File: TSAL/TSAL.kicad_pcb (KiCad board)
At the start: 2 copper layers, 89.4 x 58.2 mm, 58 parts, among them J1 Conn_02x03_Counter_Clockwise, J2 Conn_01x02, J3 Conn_02x01, J4 Conn_02x01, Q1 BSS138, Q2 BSS138, Q3 AO3401A, U1 LM358, U10 74HC74, U2 74HC27, U3 74HC20, U4 4N35, U5 74HC08, U6 74HC86, U7 LM7805_TO220, U8 LM339, U9 LM339

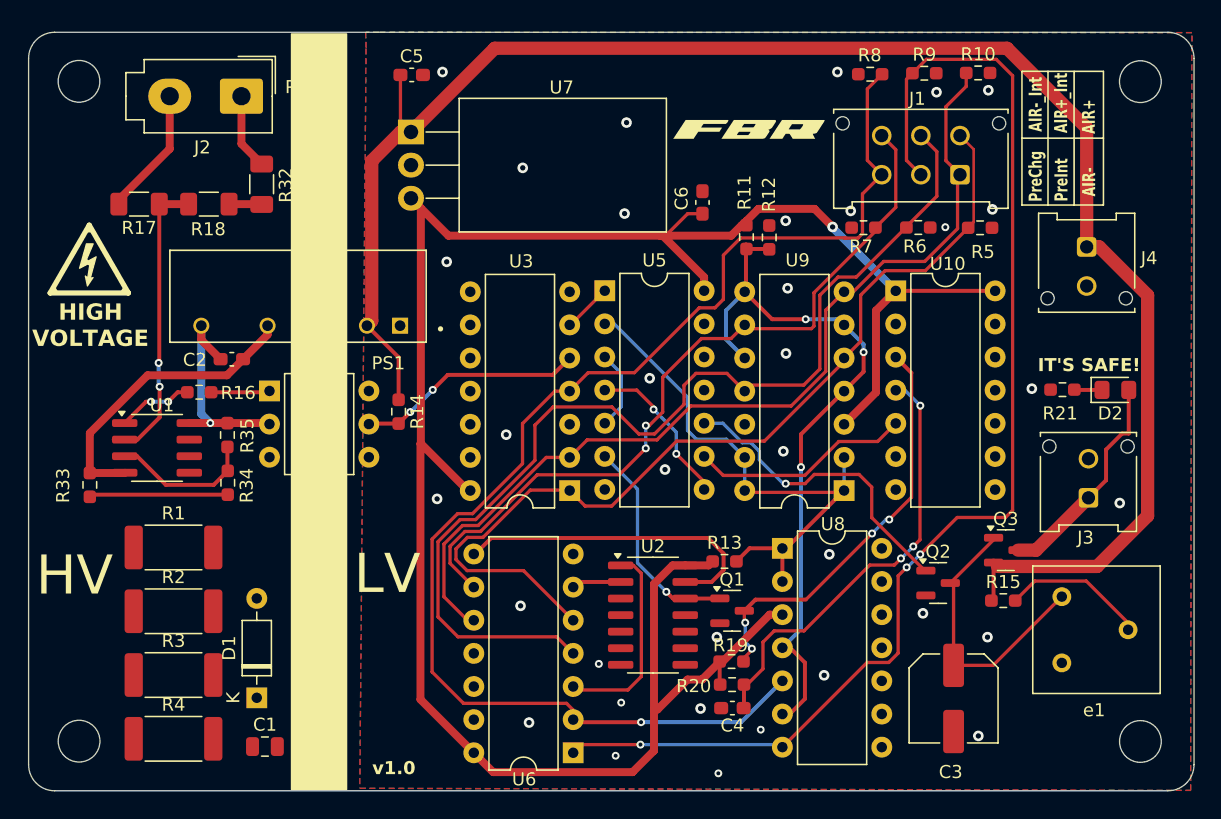
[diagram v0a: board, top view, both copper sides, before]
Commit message: minor changes
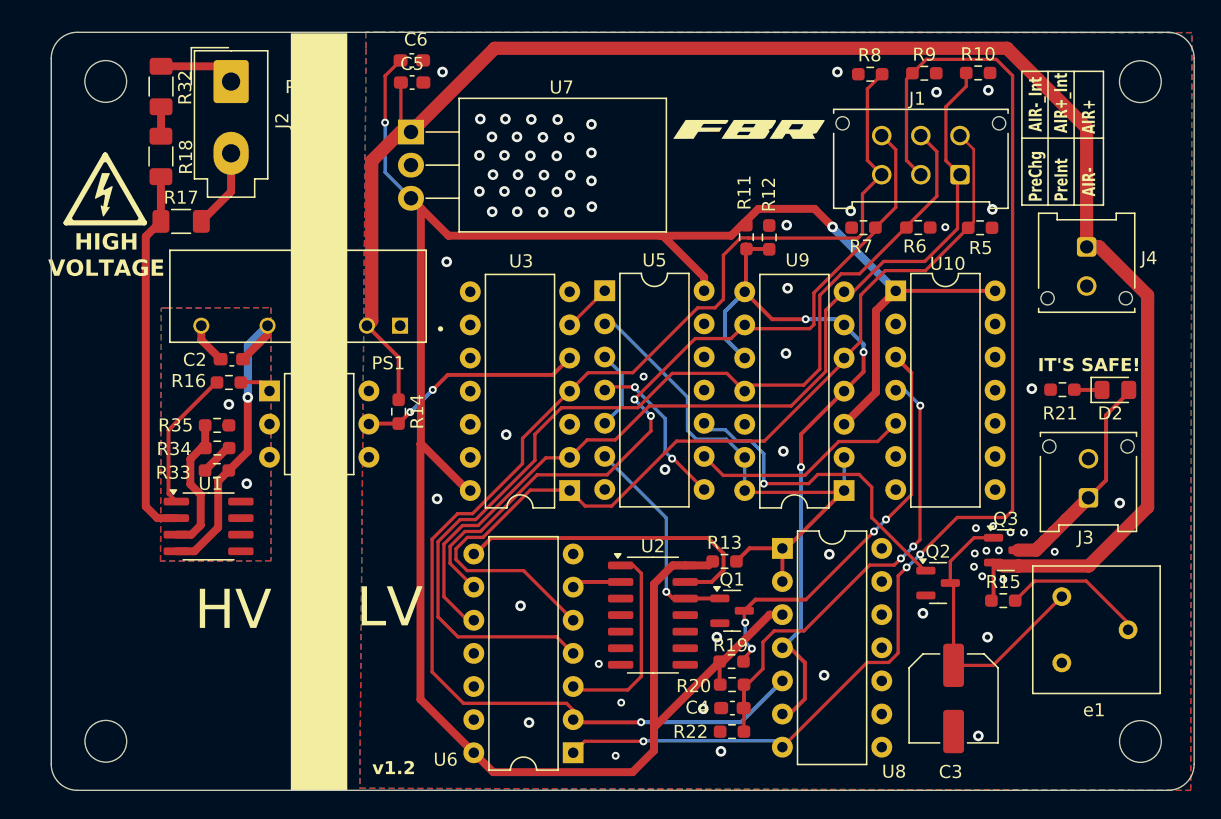
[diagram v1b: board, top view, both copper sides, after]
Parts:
- removed C1: 0.1 uF, Capacitor_SMD:C_0805_2012Metric
- removed D1: 2.4V, Diode_THT:D_DO-35_SOD27_P7.62mm_Horizontal
- removed R1, R2: 5.6K, Resistor_SMD:R_2512_6332Metric_Pad1.40x3.35mm_HandSolder
- removed R3: 6.8K, Resistor_SMD:R_2512_6332Metric_Pad1.40x3.35mm_HandSolder
- removed R4: 2.7K, Resistor_SMD:R_2512_6332Metric_Pad1.40x3.35mm_HandSolder
- added R22: 500K, Resistor_SMD:R_0603_1608Metric_Pad0.98x0.95mm_HandSolder, F.Cu at (112.4, 84.4)
- R16: value 500 -> 390
- moved C6 24.8 mm to (87.8, 33.0), turned to 180 degrees
- moved R32 10.8 mm to (68.6, 35.0)
- moved R33 9.80 mm to (72.9, 64.4), turned to 180 degrees
- moved U1 7.20 mm to (72.3, 68.7)
- moved REF** 5.52 mm to (64.3, 42.8)
- moved R18 5.18 mm to (68.6, 40.3), turned to 90 degrees
- moved R17 3.49 mm to (70.2, 45.3), turned to 0 degrees
- moved R34 2.78 mm to (72.9, 62.7), turned to 180 degrees
- moved R16 2.40 mm to (73.8, 57.7)
- moved H2 2.05 mm to (64.4, 85.2)
- moved H1 2.05 mm to (64.4, 34.6)
- moved J2 1.37 mm to (74.0, 34.6), turned to 0 degrees
- moved R35 1.08 mm to (72.9, 61.0), turned to 0 degrees
- moved C5 0.58 mm to (87.9, 34.7)
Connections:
- net HV+ renamed /HV+
- U10 pad 10: unconnected-(U10B-~{S}-Pad10) -> (no net)
- U10 pad 11: unconnected-(U10B-C-Pad11) -> (no net)
- U10 pad 12: unconnected-(U10B-D-Pad12) -> (no net)
- U10 pad 13: unconnected-(U10B-~{R}-Pad13) -> (no net)
- U10 pad 8: unconnected-(U10B-~{Q}-Pad8) -> (no net)
- U10 pad 9: unconnected-(U10B-Q-Pad9) -> (no net)
- U2 pad 10: unconnected-(U2-Pad10) -> (no net)
- U2 pad 11: unconnected-(U2-Pad11) -> (no net)
- U2 pad 9: unconnected-(U2-Pad9) -> (no net)
- U3 pad 10: unconnected-(U3-Pad10) -> (no net)
- U3 pad 12: unconnected-(U3-Pad12) -> (no net)
- U3 pad 13: unconnected-(U3-Pad13) -> (no net)
- U3 pad 8: unconnected-(U3-Pad8) -> (no net)
- U3 pad 9: unconnected-(U3-Pad9) -> (no net)
- U6 pad 11: unconnected-(U6-Pad11) -> (no net)
- U6 pad 12: unconnected-(U6-Pad12) -> (no net)
- U6 pad 13: unconnected-(U6-Pad13) -> (no net)
- U8 pad 10: unconnected-(U8C---Pad10) -> (no net)
- U8 pad 11: unconnected-(U8C-+-Pad11) -> (no net)
- U8 pad 13: unconnected-(U8-Pad13) -> (no net)
- U8 pad 14: unconnected-(U8-Pad14) -> (no net)
- U8 pad 8: unconnected-(U8D---Pad8) -> (no net)
- U8 pad 9: unconnected-(U8D-+-Pad9) -> (no net)
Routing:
- net /5V-_Iso: track 17.1 -> 3.68 mm, vias 1 -> 2
- net /5V: track 168.8 -> 179.5 mm, vias 1 -> 2
- net Net-(R33-Pad2): track 10.7 -> 2.57 mm
- net Net-(U1A--): track 22.9 -> 28.5 mm, vias 2 -> 0
- net Net-(R16-Pad1): track 5.78 -> 11.0 mm, vias 2 -> 0
- net /HV+: track 9.89 -> 6.16 mm
- net /AIR+_Int: track 80.3 -> 77.3 mm
- net /VHI<60V: track 4.83 -> 2.45 mm
- net Net-(U10A-~{S}): track 33.8 -> 35.6 mm
- net /5V+_Iso: track 23.2 -> 24.4 mm, vias 0 -> 1
- net Net-(Q2-G): track 24.0 -> 25.0 mm
- net Net-(Q2-D): track 21.7 -> 22.6 mm
- net /Precharge: track 101.2 -> 100.6 mm
- net /AIR-_Int: track 59.4 -> 59.9 mm
- net GLV-: vias 35 -> 70
- added copper zone on B.Cu, net /5V-_Iso
- added copper zone on F.Cu, net /5V-_Iso
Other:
- board size 89.4 x 58.2 mm -> 87.6 x 58.1 mm
- board text added: "87.6300 mm x 58.1200 mm"
- board text added: "v1.2"
- board text removed: "89.3550 mm x 58.1550 mm"
- board text removed: "v1.0"
